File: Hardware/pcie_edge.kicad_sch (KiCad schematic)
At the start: 1 part, among them J1 Bus_PCI_Express_x1

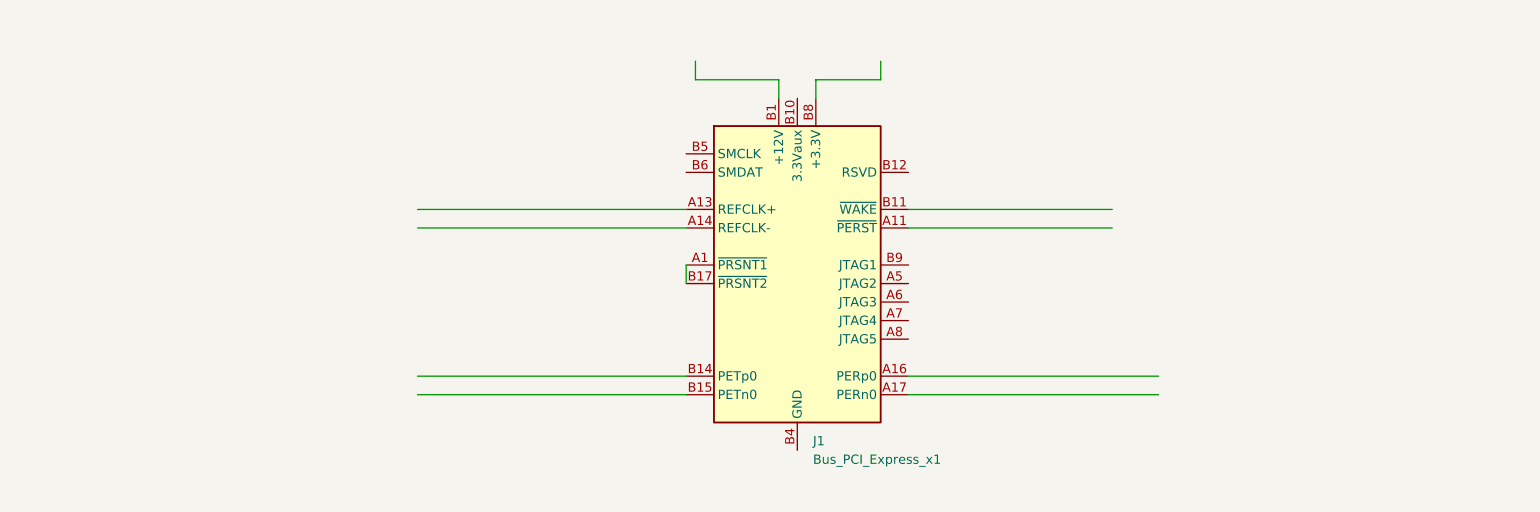
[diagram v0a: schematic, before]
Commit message: Trying to assign MGT lanes but I don't know how to do inter sheet connectivity yet
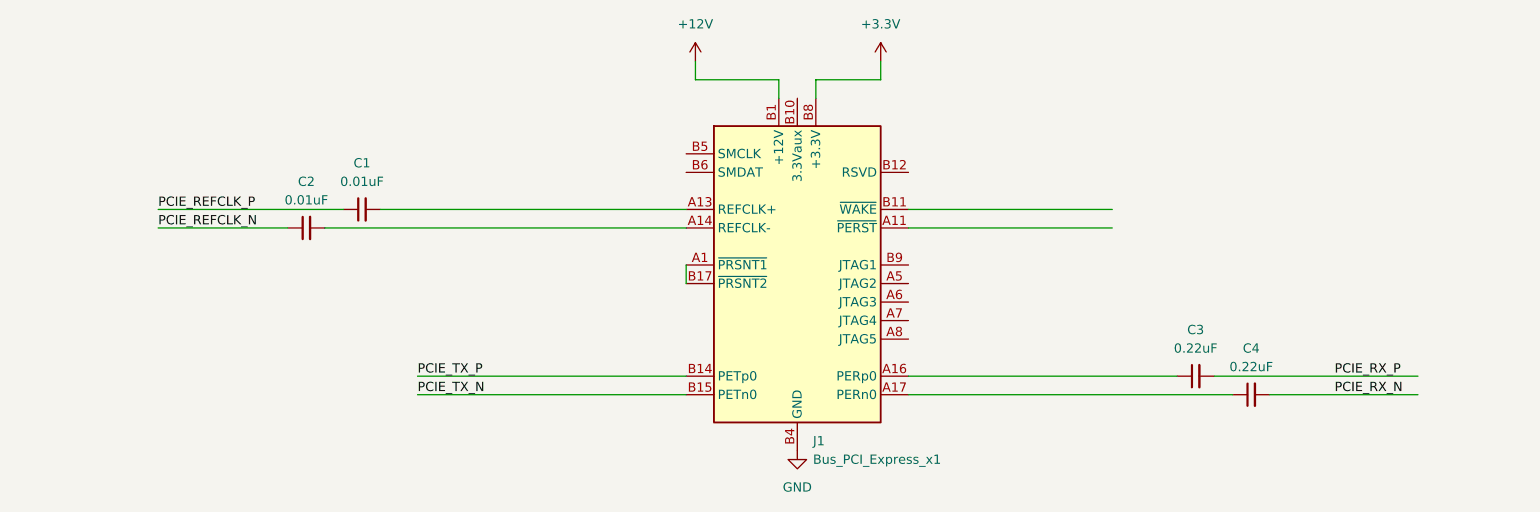
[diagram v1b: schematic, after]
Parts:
- added C1, C2: 0.01uF, Capacitor_SMD:C_0402_1005Metric, symbol Device:C_Small
- added C3, C4: 0.22uF, Capacitor_SMD:C_0402_1005Metric, symbol Device:C_Small
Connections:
- net +3.3V: now reaches J1.A10 (+3.3V), J1.A9 (+3.3V), J1.B8 (+3.3V)
- net GND: now reaches J1.A12 (GND), J1.A15 (GND), J1.A18 (GND), J1.A4 (GND), J1.B13 (GND), J1.B16 (GND), J1.B18 (GND), J1.B4 (GND), J1.B7 (GND)
- net at J1.A13 (REFCLK+): now also C1.2
- net at J1.A14 (REFCLK-): now also C2.2
- net at J1.A16 (PERp0): now also C3.1
- net at J1.A17 (PERn0): now also C4.1
- net +12V: now reaches J1.A2 (+12V), J1.A3 (+12V), J1.B1 (+12V), J1.B2 (+12V), J1.B3 (+12V)
- net PCIE_TX_P: now reaches J1.B14 (PETp0)
- net PCIE_TX_N: now reaches J1.B15 (PETn0)
- new net PCIE_REFCLK_N: C2.1
- new net PCIE_REFCLK_P: C1.1
- new net PCIE_RX_N: C4.2
- new net PCIE_RX_P: C3.2

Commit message: Found the global labels
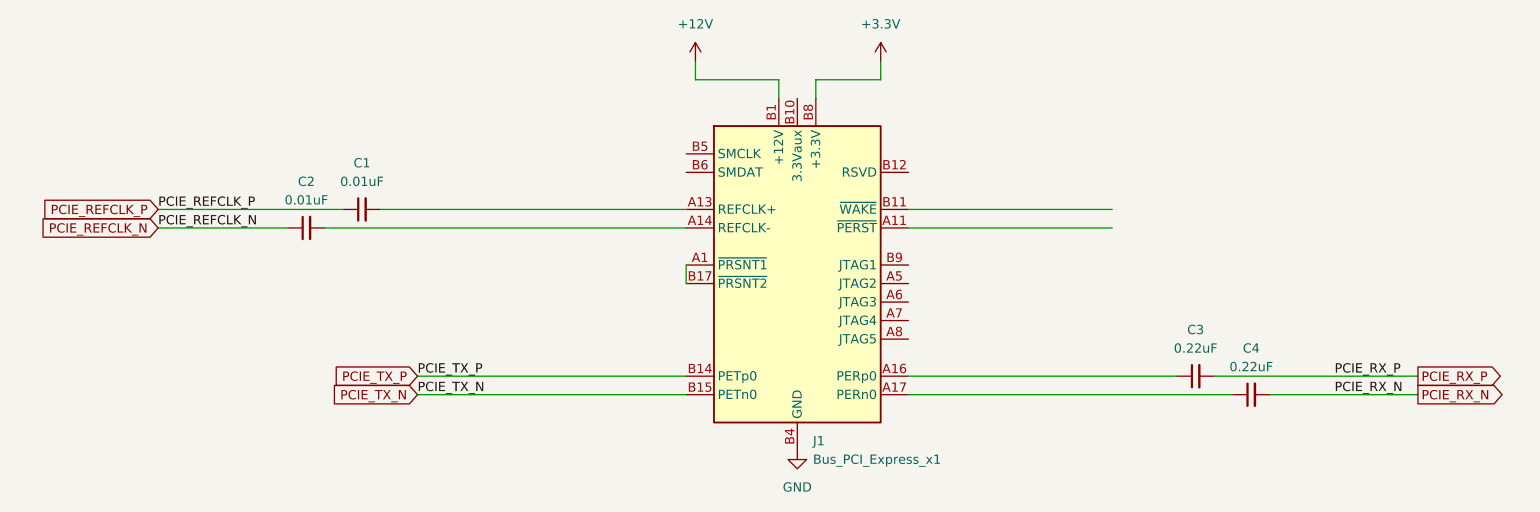
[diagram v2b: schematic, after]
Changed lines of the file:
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@@
+		)
+	)
+	(global_label "PCIE_RX_N"
+		(shape output)
+		(at 226.06 107.95 0)
+		(fields_autoplaced yes)
+		(effects
+			(font
+				(size 1.27 1.27)
+			)
+			(justify left)
+		)
+		(property "Intersheetrefs" "${INTERSHEET_REFS}"
+			(at 239.0842 107.95 0)
+			(hide yes)
+			(show_name no)
+			(do_not_autoplace no)
+			(effects
+				(font
+					(size 1.27 1.27)
+				)
+				(justify left)
+			)
+		)
+	)
+	(global_label "PCIE_REFCLK_N"
+		(shape input)
+		(at 53.34 85.09 180)
+		(fields_autoplaced yes)
+		(effects
+			(font
+				(size 1.27 1.27)
+			)
+			(justify right)
+		)
+		(property "Intersheetrefs" "${INTERSHEET_REFS}"
+			(at 35.7196 85.09 0)
+			(hide yes)
+			(show_name no)
+			(do_not_autoplace no)
+			(effects
+				(font
+					(size 1.27 1.27)
+				)
+				(justify right)
+			)
+		)
+	)
+	(global_label "PCIE_RX_P"
+		(shape output)
+		(at 226.06 105.41 0)
+		(fields_autoplaced yes)
+		(effects
+			(font
+				(size 1.27 1.27)
+			)
+			(justify left)
+		)
+		(property "Intersheetrefs" "${INTERSHEET_REFS}"
+			(at 239.0237 105.41 0)
+			(hide yes)
+			(show_name no)
+			(do_not_autoplace no)
+			(effects
+				(font
+					(size 1.27 1.27)
+				)
+				(justify left)
+			)
+		)
+	)
+	(global_label "PCIE_REFCLK_P"
+		(shape input)
+		(at 53.34 82.55 180)
+		(fields_autoplaced yes)
+		(effects
+			(font
+				(size 1.27 1.27)
+			)
+			(justify right)
+		)
+		(property "Intersheetrefs" "${INTERSHEET_REFS}"
+			(at 35.7801 82.55 0)
+			(hide yes)
+			(show_name no)
+			(do_not_autoplace no)
+			(effects
+				(font
+					(size 1.27 1.27)
+				)
+				(justify right)
+			)
+		)
+	)
+	(global_label "PCIE_TX_N"
+		(shape input)
+		(at 88.9 107.95 180)
+		(fields_autoplaced yes)
+		(effects
+			(font
+				(size 1.27 1.27)
+			)
+			(justify right)
+		)
+		(property "Intersheetrefs" "${INTERSHEET_REFS}"
+			(at 76.1782 107.95 0)
+			(hide yes)
+			(show_name no)
+			(do_not_autoplace no)
+			(effects
+				(font
+					(size 1.27 1.27)
+				)
+				(justify right)
+			)
+		)
+	)
+	(global_label "PCIE_TX_P"
+		(shape input)
+		(at 88.9 105.41 180)
+		(fields_autoplaced yes)
+		(effects
+			(font
+				(size 1.27 1.27)
+			)
+			(justify right)
+		)
+		(property "Intersheetrefs" "${INTERSHEET_REFS}"
+			(at 76.2387 105.41 0)
+			(hide yes)
+			(show_name no)
+			(do_not_autoplace no)
+			(effects
+				(font
+					(size 1.27 1.27)
+				)
+				(justify right)
+			)
 		)
 	)
